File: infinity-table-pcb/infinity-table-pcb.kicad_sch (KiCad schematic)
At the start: 15 parts, among them J1 PJ-063AH, J2 Conn_01x04_Male, J3 Conn_01x10_Male, SW1 SW_Push_Dual, SW2 SW_Push_Dual, U1 TXS0108EPW

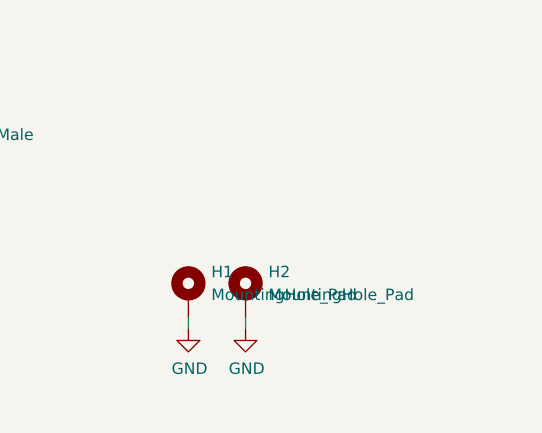
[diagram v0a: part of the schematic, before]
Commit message: moar holes
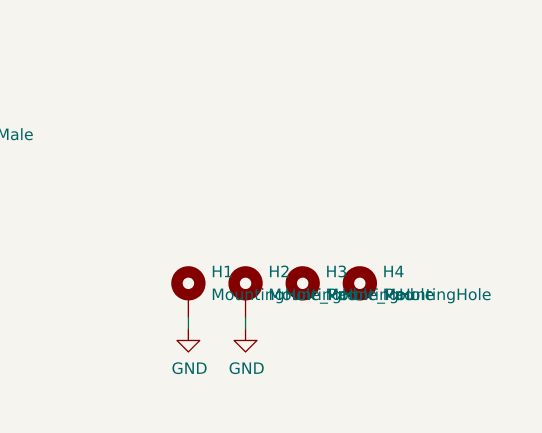
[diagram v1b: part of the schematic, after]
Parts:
- added H3, H4: MountingHole, MountingHole:MountingHole_2.2mm_M2, symbol Mechanical:MountingHole
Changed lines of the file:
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@@
     (pin "1")
+  )
+  (symbol (lib_id "Mechanical:MountingHole") (at 260.35 139.7 0) (unit 1)
+    (in_bom yes) (on_board yes) (fields_autoplaced)
+    (property "Reference" "H4" (id 0) (at 262.89 138.4299 0)
+      (effects (font (size 1.27 1.27)) (justify left))
+    )
+    (property "Value" "MountingHole" (id 1) (at 262.89 140.9699 0)
+      (effects (font (size 1.27 1.27)) (justify left))
+    )
+    (property "Footprint" "MountingHole:MountingHole_2.2mm_M2" (id 2) (at 260.35 139.7 0)
+      (effects (font (size 1.27 1.27)) hide)
+    )
+    (property "Datasheet" "~" (id 3) (at 260.35 139.7 0)
+      (effects (font (size 1.27 1.27)) hide)
+    )
   )
   (symbol (lib_id "Mechanical:MountingHole_Pad") (at 247.65 140.97 0) (unit 1)
@@
     )
     (pin "1")
+  )
+  (symbol (lib_id "Mechanical:MountingHole") (at 254 139.7 0) (unit 1)
+    (in_bom yes) (on_board yes) (fields_autoplaced)
+    (property "Reference" "H3" (id 0) (at 256.54 138.4299 0)
+      (effects (font (size 1.27 1.27)) (justify left))
+    )
+    (property "Value" "MountingHole" (id 1) (at 256.54 140.9699 0)
+      (effects (font (size 1.27 1.27)) (justify left))
+    )
+    (property "Footprint" "MountingHole:MountingHole_2.2mm_M2" (id 2) (at 254 139.7 0)
+      (effects (font (size 1.27 1.27)) hide)
+    )
+    (property "Datasheet" "~" (id 3) (at 254 139.7 0)
+      (effects (font (size 1.27 1.27)) hide)
+    )
   )
   (symbol (lib_id "power:GND") (at 247.65 144.78 0) (unit 1)
@@
       (reference "H2") (unit 1) (value "MountingHole_Pad") (footprint "MountingHole:MountingHole_4.3mm_M4_Pad")
     )
+    (path "/65fd9534-1b91-42a6-8ecd-7a42d8ae4ade"
+      (reference "H3") (unit 1) (value "MountingHole") (footprint "MountingHole:MountingHole_2.2mm_M2")
+    )
+    (path "/28d92791-e03b-49b7-ab76-0b79e48b37f2"
+      (reference "H4") (unit 1) (value "MountingHole") (footprint "MountingHole:MountingHole_2.2mm_M2")
+    )
     (path "/00000000-0000-0000-0000-00005bf7fa3a"
